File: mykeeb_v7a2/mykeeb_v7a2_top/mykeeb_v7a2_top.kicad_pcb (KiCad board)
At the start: 2 copper layers, 160.4 x 128.9 mm, 9 parts

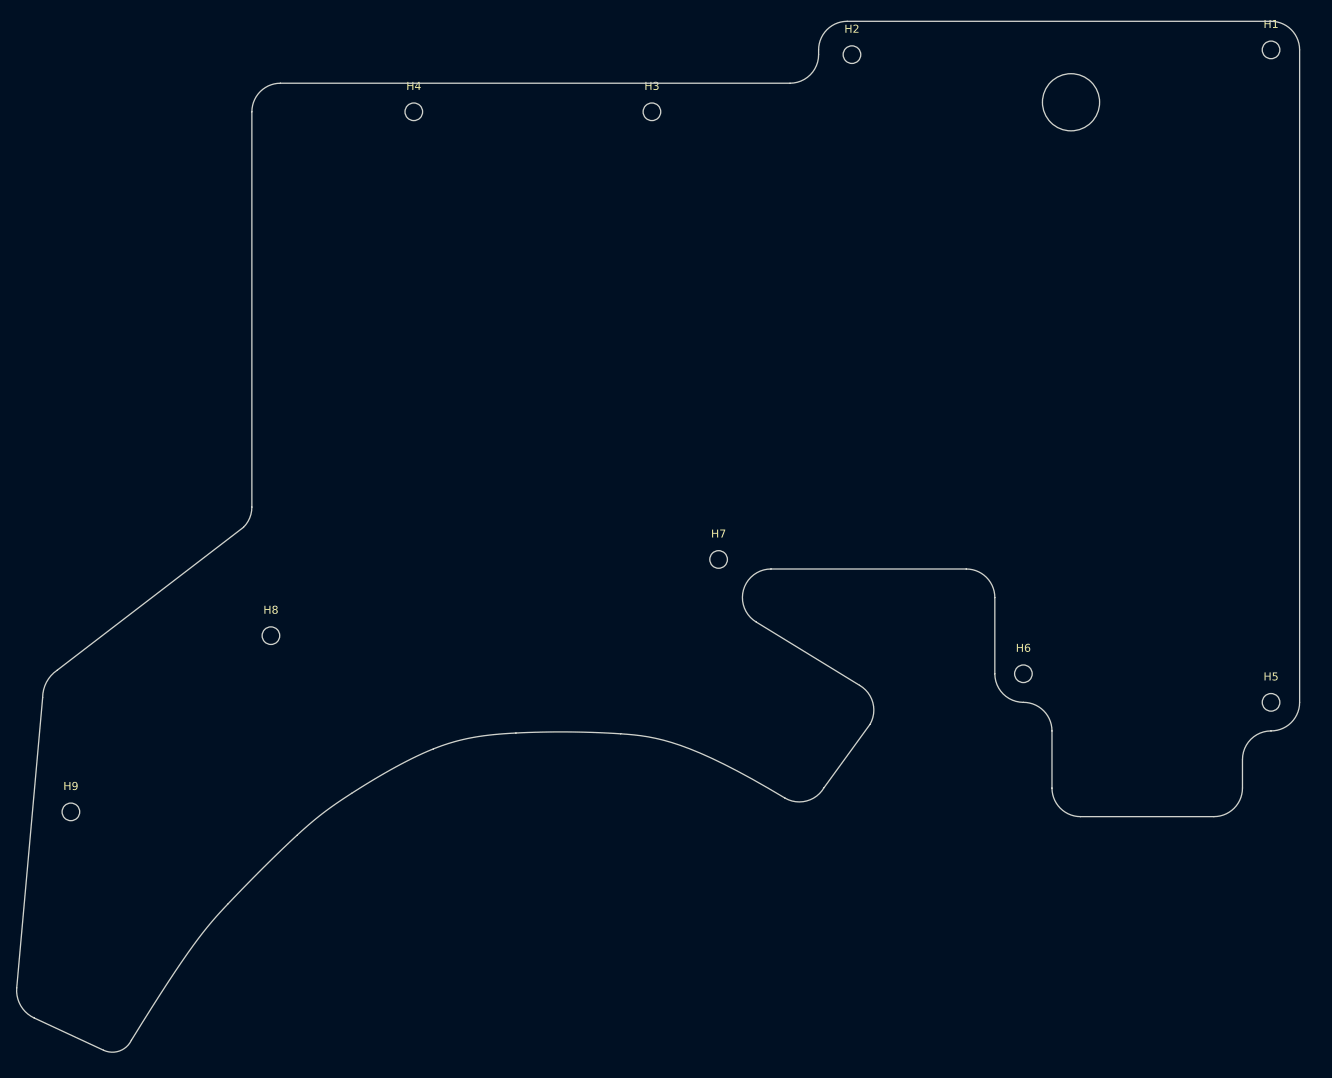
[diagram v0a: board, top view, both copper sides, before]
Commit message: add gerber files for v7a2
Signed-off-by: Maximilian Huber <gh@maxhbr.de>
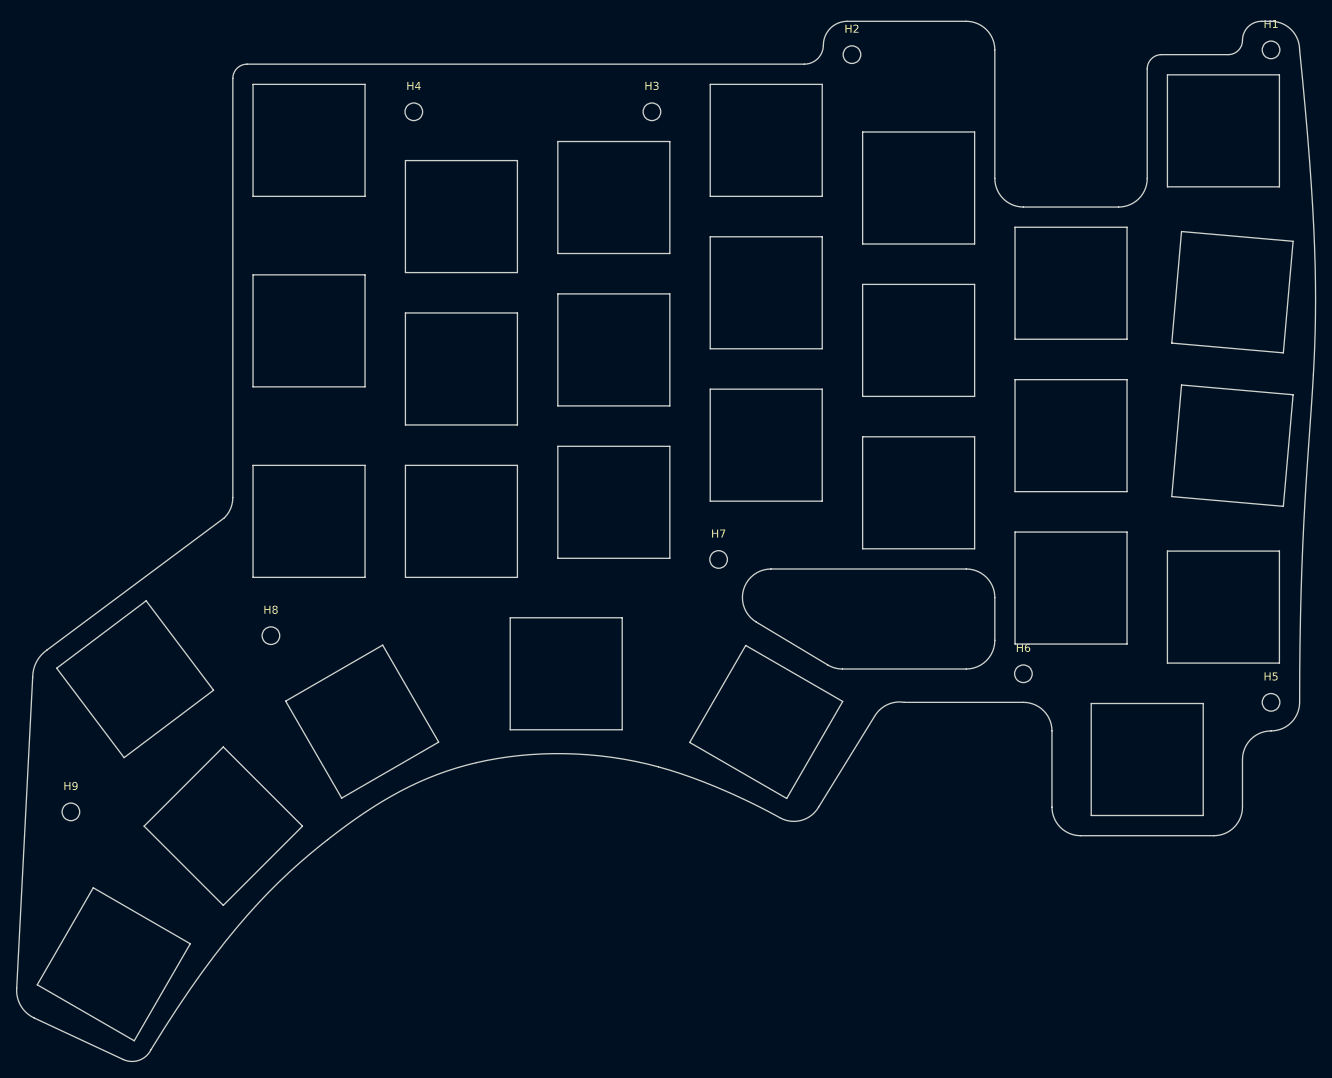
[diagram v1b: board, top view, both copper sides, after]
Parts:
- added S0: SW, pretty:SW_Hole, F.Cu at (171.5, 163.1)
- added S10: SW, pretty:SW_Hole, F.Cu at (172.6, 183.3)
- added S11: SW, pretty:SW_Hole, F.Cu at (152.4, 182.2)
- added S12: SW, pretty:SW_Hole, F.Cu at (133.4, 170.3)
- added S13: SW, pretty:SW_Hole, F.Cu at (114.3, 164.3)
- added S14: SW, pretty:SW_Hole, F.Cu at (95.3, 171.5)
- added S15: SW, pretty:SW_Hole, F.Cu at (76.2, 173.8)
- added S2: SW, pretty:SW_Hole, F.Cu at (57.2, 164.3)
- added S20: SW, pretty:SW_Hole, F.Cu at (172.6, 202.5)
- added S21: SW, pretty:SW_Hole, F.Cu at (152.4, 201.2)
- added S22: SW, pretty:SW_Hole, F.Cu at (133.4, 189.3)
- added S23: SW, pretty:SW_Hole, F.Cu at (114.3, 183.4)
- added S24: SW, pretty:SW_Hole, F.Cu at (95.3, 190.5)
- added S25: SW, pretty:SW_Hole, F.Cu at (76.2, 192.9)
- added S3: SW, pretty:SW_Hole, F.Cu at (57.2, 188.1)
- added S30: SW, pretty:SW_Hole, F.Cu at (171.5, 222.6)
- added S31: SW, pretty:SW_Hole, F.Cu at (152.4, 220.3)
- added S32: SW, pretty:SW_Hole, F.Cu at (133.4, 208.4)
- added S33: SW, pretty:SW_Hole, F.Cu at (114.3, 202.4)
- added S34: SW, pretty:SW_Hole, F.Cu at (95.3, 209.6)
- added S35: SW, pretty:SW_Hole, F.Cu at (76.2, 211.9)
- added S4: SW, pretty:SW_Hole, F.Cu at (57.1, 211.9)
- added S40: SW, pretty:SW_Hole, F.Cu at (161.9, 241.7)
- added S42: SW, pretty:SW_Hole, F.Cu at (89.3, 231.0)
- added S43: SW, pretty:SW_Hole, F.Cu at (63.8, 237.0)
- added S44: SW, pretty:SW_Hole, F.Cu at (46.4, 250.0)
- added S5: SW, pretty:SW_Hole, F.Cu at (35.4, 231.7)
- added locked: SW, pretty:SW_Hole, F.Cu at (32.7, 267.3)
- added locked: SW, pretty:SW_Hole, F.Cu at (114.3, 237.0)
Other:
- board size 160.4 x 128.9 mm -> 162.4 x 130 mm
